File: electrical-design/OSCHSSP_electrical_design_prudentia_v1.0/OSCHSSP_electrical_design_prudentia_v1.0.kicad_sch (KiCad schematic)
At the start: 22 parts, among them J1 Mains 120V 60Hz 15Amax, J2 LCD-I2C, J3 SD-I2C, SW1 SW_DIP_x01, SW2 RotaryEncoder_Switch, U1 34.81-9024, U1 MAX31855, U2 34.81-9024

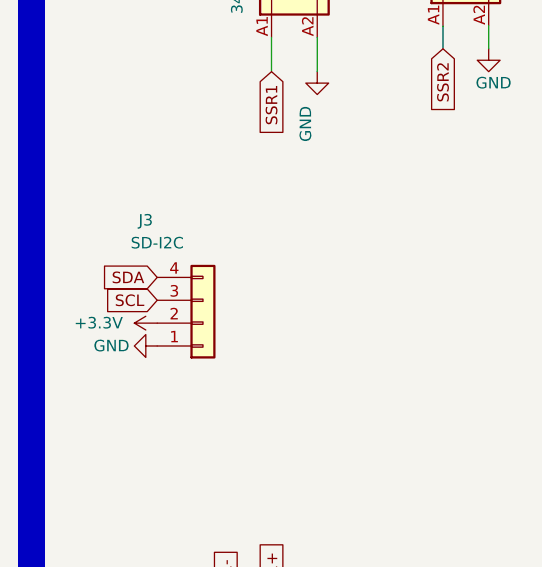
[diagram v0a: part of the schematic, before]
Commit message: updated and organized files
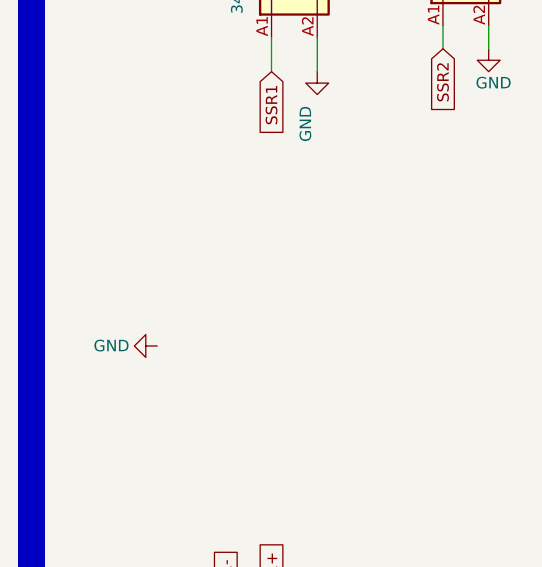
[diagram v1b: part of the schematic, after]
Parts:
- removed J3: SD-I2C, Connector_PinSocket_2.54mm:PinSocket_1x04_P2.54mm_Horizontal, symbol Connector_Generic:Conn_01x04
